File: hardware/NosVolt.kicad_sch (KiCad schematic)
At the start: 18 parts, among them J101 INPUTS, J102 OUTPUTS, SW101 SW_Reset, SW102 SSSS811101, U101 GMT028-05, U102 ESP32-S3-WROOM-1

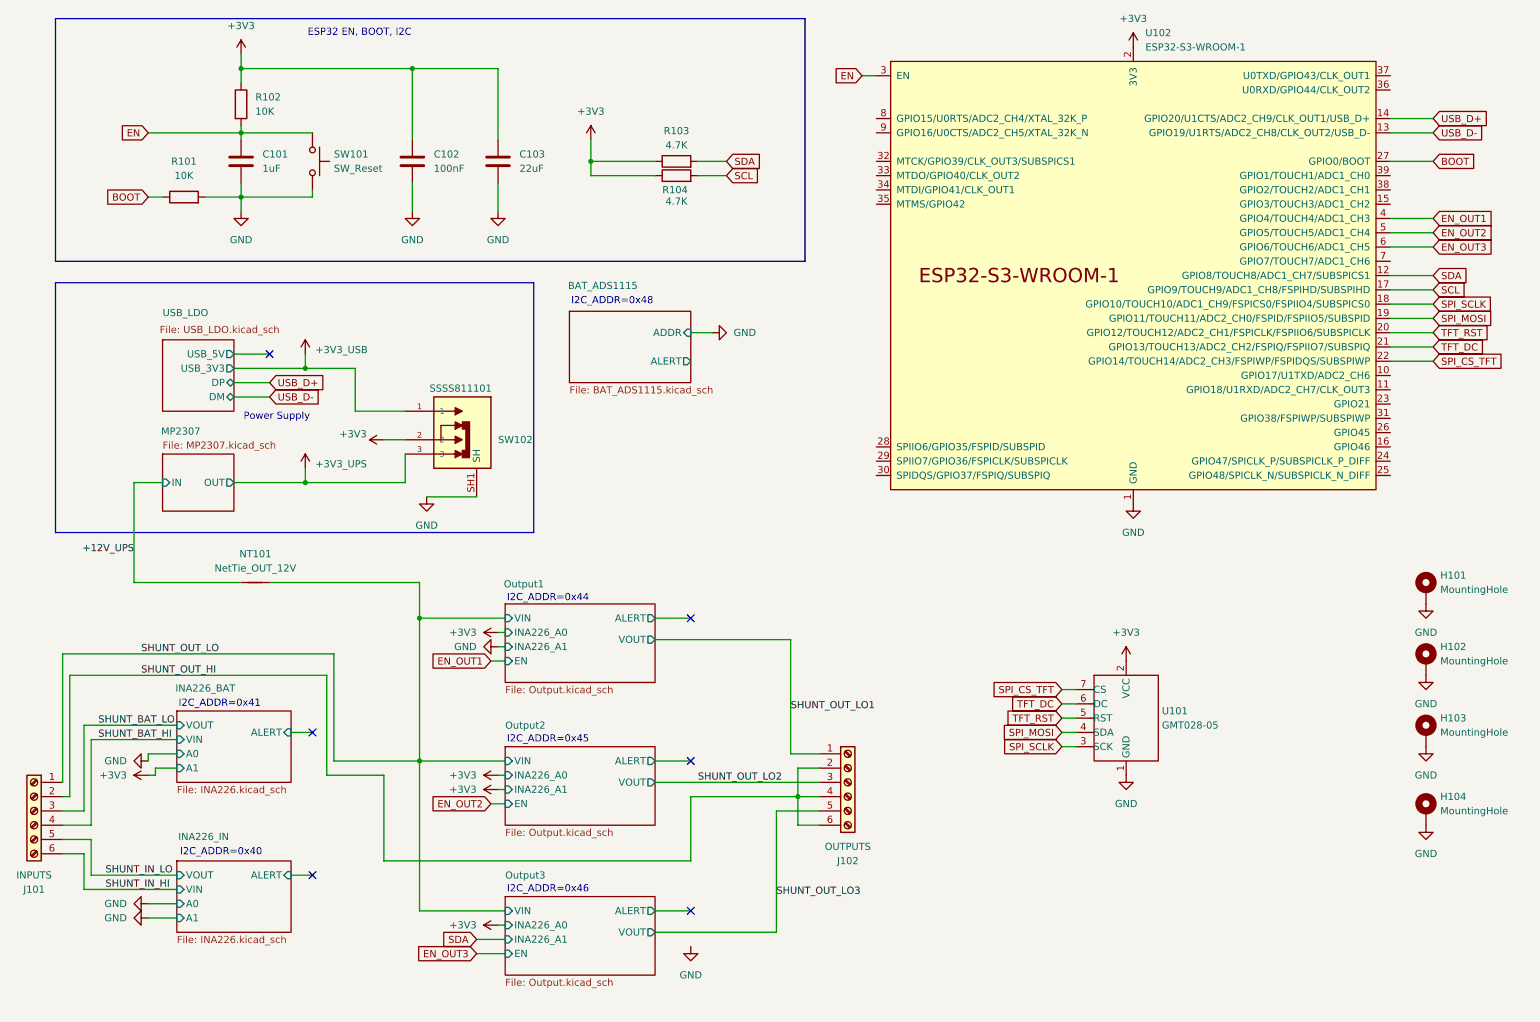
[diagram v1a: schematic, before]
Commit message: Test points
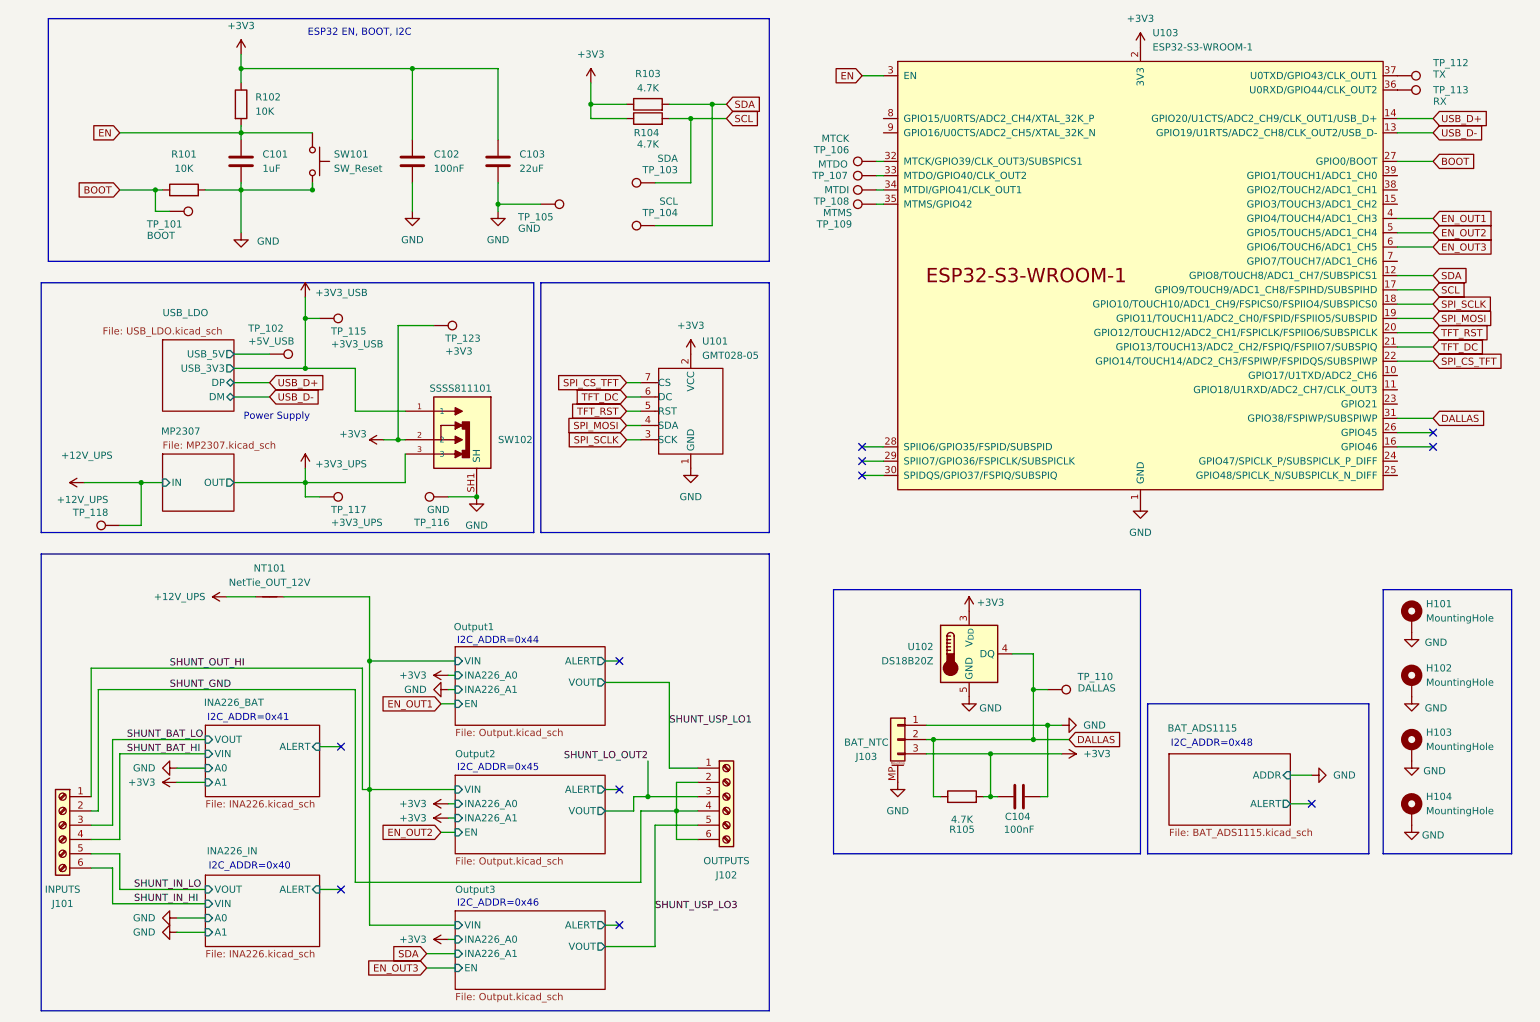
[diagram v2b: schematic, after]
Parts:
- added C104: 100nF, Capacitor_SMD:C_0603_1608Metric, symbol Device:C
- added J103: BAT_NTC, Connector_JST:JST_GH_SM03B-GHS-TB_1x03-1MP_P1.25mm_Horizontal, symbol Connector_Generic_MountingPin:Conn_01x03_MountingPin
- added R105: 4.7K, Resistor_SMD:R_0603_1608Metric_Pad0.98x0.95mm_HandSolder, symbol Device:R
- added TP_101: BOOT, NosLib:TestPoint_Pad_1.0x1.0mm, symbol Connector:TestPoint
- added TP_102: +5V_USB, NosLib:TestPoint_Pad_1.0x1.0mm, symbol Connector:TestPoint
- added TP_103: SDA, NosLib:TestPoint_Pad_1.0x1.0mm, symbol Connector:TestPoint
- added TP_104: SCL, NosLib:TestPoint_Pad_1.0x1.0mm, symbol Connector:TestPoint
- added TP_105, TP_116: GND, NosLib:TestPoint_Pad_1.0x1.0mm, symbol Connector:TestPoint
- added TP_106: MTCK, NosLib:TestPoint_Pad_1.0x1.0mm, symbol Connector:TestPoint
- added TP_107: MTDO, NosLib:TestPoint_Pad_1.0x1.0mm, symbol Connector:TestPoint
- added TP_108: MTDI, NosLib:TestPoint_Pad_1.0x1.0mm, symbol Connector:TestPoint
- added TP_109: MTMS, NosLib:TestPoint_Pad_1.0x1.0mm, symbol Connector:TestPoint
- added TP_110: DALLAS, NosLib:TestPoint_Pad_1.0x1.0mm, symbol Connector:TestPoint
- added TP_112: TX, NosLib:TestPoint_Pad_1.0x1.0mm, symbol Connector:TestPoint
- added TP_113: RX, NosLib:TestPoint_Pad_1.0x1.0mm, symbol Connector:TestPoint
- added TP_115: +3V3_USB, NosLib:TestPoint_Pad_1.0x1.0mm, symbol Connector:TestPoint
- added TP_117: +3V3_UPS, NosLib:TestPoint_Pad_1.0x1.0mm, symbol Connector:TestPoint
- added TP_118: +12V_UPS, NosLib:TestPoint_Pad_1.0x1.0mm, symbol Connector:TestPoint
- added TP_123: +3V3, NosLib:TestPoint_Pad_1.0x1.0mm, symbol Connector:TestPoint
- added U102: DS18B20Z, Package_SO:SOIC-8_3.9x4.9mm_P1.27mm, symbol Sensor_Temperature:DS18B20Z
- renumbered U102 to U103
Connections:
- net SHUNT_OUT_LO is gone; now on net SHUNT_OUT_HI: J101.1 (Pin_1), NT101.2
- net +12V_UPS: now also TP_118.1
- net +3V3: now also C104.1, J103.3 (Pin_3), R105.2, TP_123.1, U102.3 (V_{DD})
- net +3V3_UPS: now also TP_117.1
- net +3V3_USB: now also TP_115.1
- net BOOT: now also TP_101.1
- net GND: now also C104.2, J103.1 (Pin_1), J103.MP (MountPin), TP_105.1, TP_116.1, U102.5 (GND)
- net SCL: now also TP_103.1
- net SDA: now also TP_104.1
- net SHUNT_OUT_HI: no longer J101.2 (Pin_2), J102.2 (Pin_2), J102.4 (Pin_4), J102.6 (Pin_6)
- net USB_LDO/USB_5V: now also TP_102.1
- net DALLAS: now reaches U103.31 (GPIO38/FSPIWP/SUBSPIWP)
- net DALLAS: now also J103.2 (Pin_2), R105.1, TP_110.1, U102.4 (DQ)
- net at U103.32 (MTCK/GPIO39/CLK_OUT3/SUBSPICS1): now also TP_106.1
- net at U103.33 (MTDO/GPIO40/CLK_OUT2): now also TP_107.1
- net at U103.34 (MTDI/GPIO41/CLK_OUT1): now also TP_108.1
- net at U103.35 (MTMS/GPIO42): now also TP_109.1
- net at U103.36 (U0RXD/GPIO44/CLK_OUT2): now also TP_113.1
- net at U103.37 (U0TXD/GPIO43/CLK_OUT1): now also TP_112.1
- net SHUNT_OUT_LO1 renamed SHUNT_USP_LO1
- net SHUNT_OUT_LO2 renamed SHUNT_LO_OUT2
- net SHUNT_OUT_LO3 renamed SHUNT_USP_LO3
- new net SHUNT_GND: J101.2 (Pin_2), J102.2 (Pin_2), J102.4 (Pin_4), J102.6 (Pin_6)
- no-connect marks 6 -> 11
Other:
- moved on the sheet: H101, H102, H103, H104, J101, J102, NT101, R101, R103, R104, U101, U103
